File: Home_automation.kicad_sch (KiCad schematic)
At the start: 105 parts, among them Q1 BTA16-600B, Q2 BTA16-600B, Q3 BTA16-600B, Q4 BTA16-600B, Q5 BTA16-600B, Q6 BTA16-600B, SW1 SW_Push, SW2 SW_Push, U1 MOC3010M, U2 MOC3010M, U3 ESP-12E, U4 MOC3010M, U5 MOC3010M, U6 EL817, U7 MOC3010M, U8 AMS1117-3.3, U9 MOC3010M

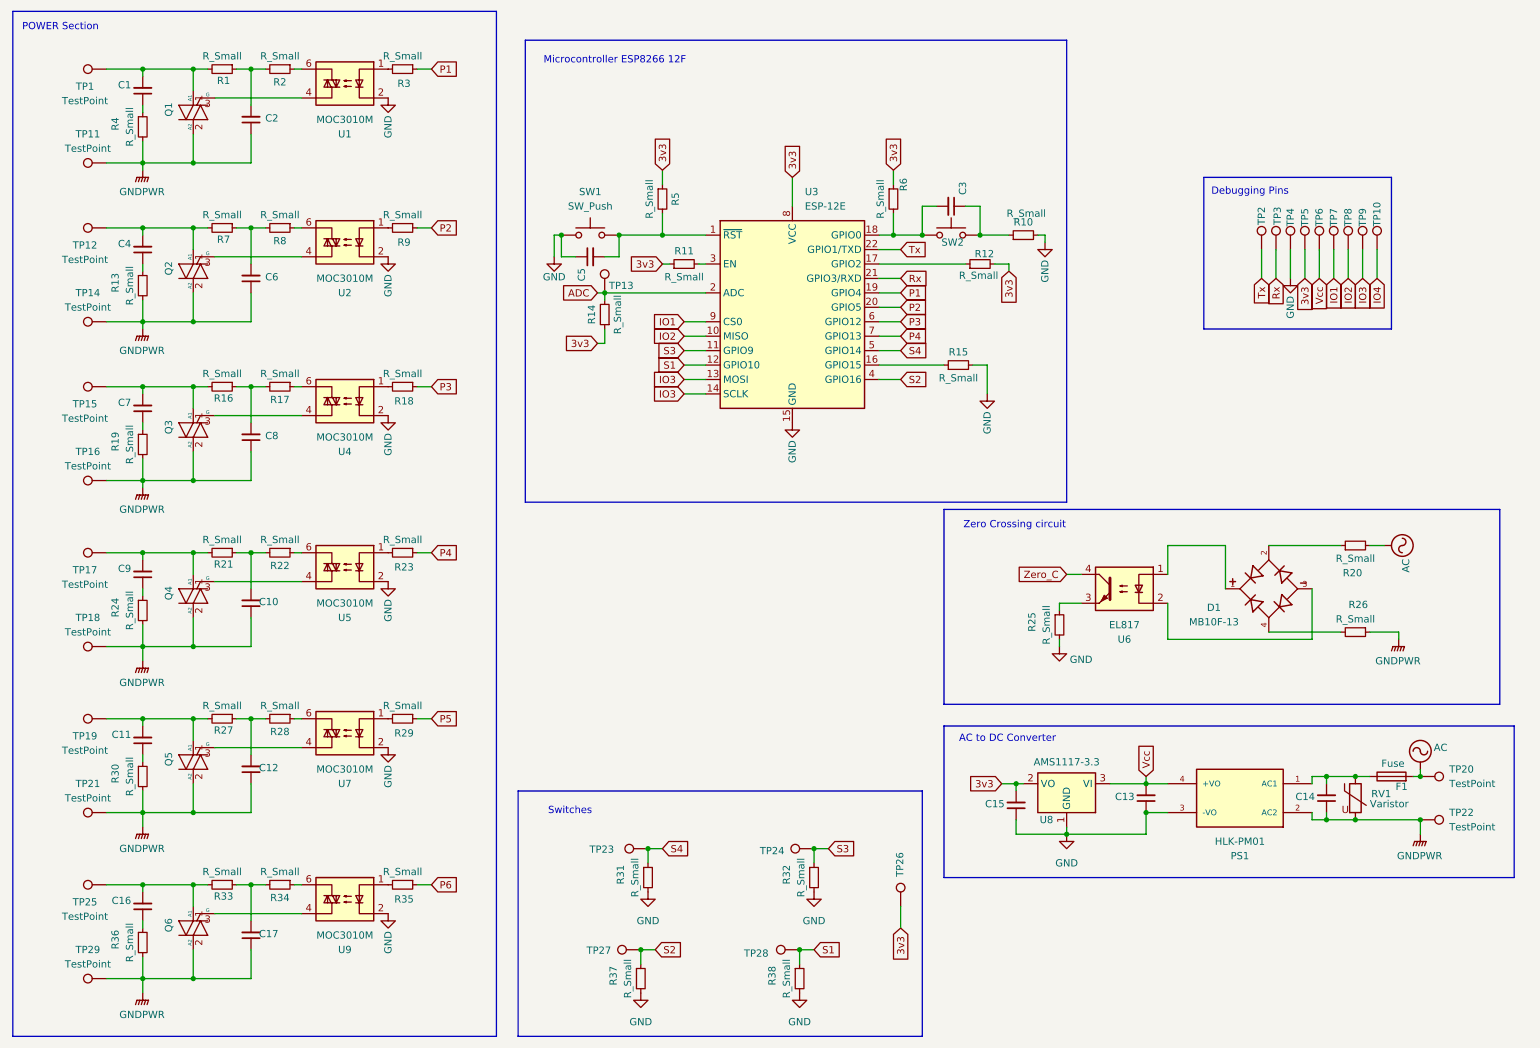
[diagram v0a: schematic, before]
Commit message: updated pcb
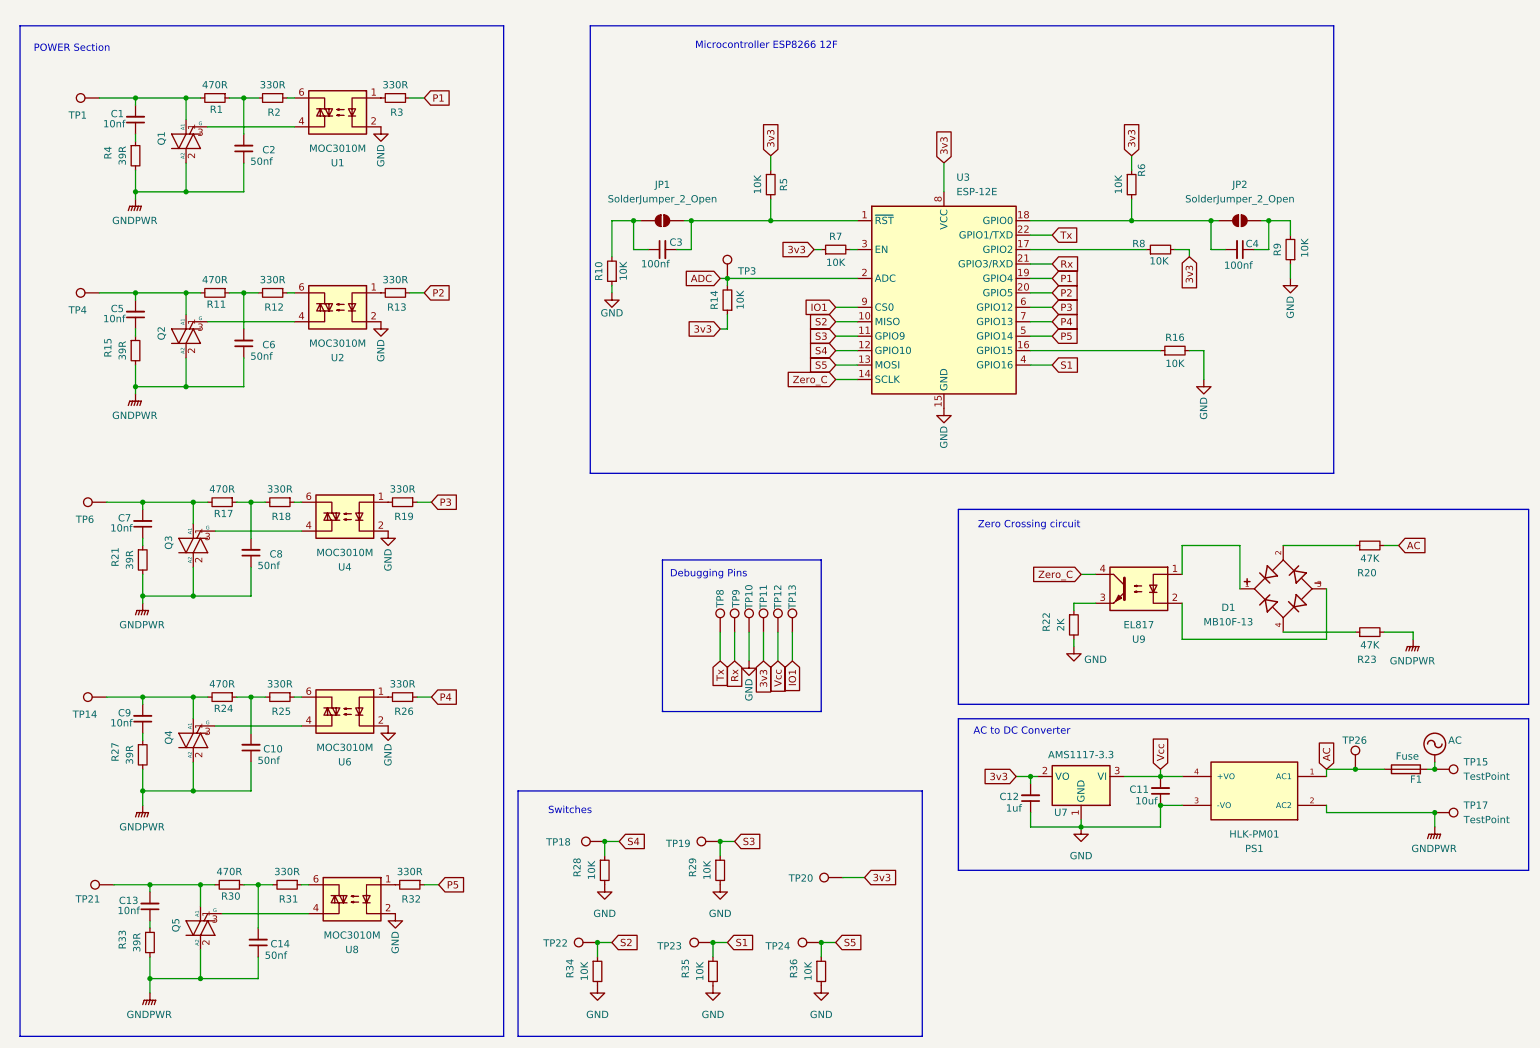
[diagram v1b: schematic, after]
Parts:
- removed C14, C16, C17, C4: C_Small, symbol Device:C_Small
- removed Q6: BTA16-600B, Package_TO_SOT_THT:TO-220-3_Vertical, symbol Triac_Thyristor:BTA16-600B
- removed R16, R22, R27, R28, R32, R37, R38, R7, R8, R9: R_Small, symbol Device:R_Small
- removed RV1: Varistor, symbol Device:Varistor
- removed SW1, SW2: SW_Push, symbol Switch:SW_Push
- removed TP10, TP11, TP14, TP16, TP18, TP21, TP25, TP29, TP8, TP9: TestPoint, symbol Connector:TestPoint
- removed U6: EL817, Package_DIP:DIP-4_W7.62mm, symbol Isolator:EL817
- removed U9: MOC3010M, symbol Relay_SolidState:MOC3010M
- added C5: 10nf, Capacitor_THT:C_Rect_L13.0mm_W3.0mm_P10.00mm_FKS3_FKP3_MKS4, symbol Device:C_Small
- added JP1, JP2: SolderJumper_2_Open, my_foot:my_foot, symbol Jumper:SolderJumper_2_Open
- added R10, R29: 10K, Resistor_SMD:R_0603_1608Metric_Pad0.98x0.95mm_HandSolder, symbol Device:R_Small
- added R11, R24: 470R, Resistor_SMD:R_0603_1608Metric_Pad0.98x0.95mm_HandSolder, symbol Device:R_Small
- added R12, R25, R31: 330R, Resistor_SMD:R_0603_1608Metric_Pad0.98x0.95mm_HandSolder, symbol Device:R_Small
- added R15: 39R, Resistor_SMD:R_0603_1608Metric_Pad0.98x0.95mm_HandSolder, symbol Device:R_Small
- added TP24, TP26: TestPoint, TestPoint:TestPoint_Loop_D3.80mm_Drill2.0mm, symbol Connector:TestPoint
- added U9: EL817, Package_DIP:DIP-4_W7.62mm, symbol Isolator:EL817
- C1, C7, C9: value C_Small -> 10nf; footprint (none) -> Capacitor_THT:C_Rect_L13.0mm_W3.0mm_P10.00mm_FKS3_FKP3_MKS4
- C10, C2, C6, C8: value C_Small -> 50nf; footprint (none) -> Capacitor_THT:C_Rect_L13.0mm_W3.0mm_P10.00mm_FKS3_FKP3_MKS4
- C11: renamed from C13; value C_Small -> 10uf; footprint (none) -> Capacitor_SMD:C_0805_2012Metric
- C12: renamed from C15; value C_Small -> 1uf; footprint (none) -> Capacitor_SMD:C_0603_1608Metric_Pad1.08x0.95mm_HandSolder
- C13: renamed from C11; value C_Small -> 10nf; footprint (none) -> Capacitor_THT:C_Rect_L13.0mm_W3.0mm_P10.00mm_FKS3_FKP3_MKS4
- C14: renamed from C12; value C_Small -> 50nf; footprint (none) -> Capacitor_THT:C_Rect_L13.0mm_W3.0mm_P10.00mm_FKS3_FKP3_MKS4
- C3: renamed from C5; value C_Small -> 100nf; footprint (none) -> Capacitor_SMD:C_0402_1005Metric_Pad0.74x0.62mm_HandSolder
- C4: renamed from C3; value C_Small -> 100nf; footprint (none) -> Capacitor_SMD:C_0402_1005Metric_Pad0.74x0.62mm_HandSolder
- F1: footprint (none) -> Fuse:Fuseholder_Cylinder-5x20mm_Schurter_0031_8201_Horizontal_Open
- R1, R17, R30: value R_Small -> 470R; footprint (none) -> Resistor_SMD:R_0603_1608Metric_Pad0.98x0.95mm_HandSolder
- R13, R18, R19, R2, R26, R3: value R_Small -> 330R; footprint (none) -> Resistor_SMD:R_0603_1608Metric_Pad0.98x0.95mm_HandSolder
- R14, R34, R35, R36, R5, R6: value R_Small -> 10K; footprint (none) -> Resistor_SMD:R_0603_1608Metric_Pad0.98x0.95mm_HandSolder
- R16: renamed from R15; value R_Small -> 10K; footprint (none) -> Resistor_SMD:R_0603_1608Metric_Pad0.98x0.95mm_HandSolder
- R20, R23: value R_Small -> 47K; footprint (none) -> Resistor_SMD:R_0603_1608Metric_Pad0.98x0.95mm_HandSolder
- R21, R33, R4: value R_Small -> 39R; footprint (none) -> Resistor_SMD:R_0603_1608Metric_Pad0.98x0.95mm_HandSolder
- R22: renamed from R25; value R_Small -> 2K; footprint (none) -> Resistor_SMD:R_0603_1608Metric_Pad0.98x0.95mm_HandSolder
- R27: renamed from R24; value R_Small -> 39R; footprint (none) -> Resistor_SMD:R_0603_1608Metric_Pad0.98x0.95mm_HandSolder
- R28: renamed from R31; value R_Small -> 10K; footprint (none) -> Resistor_SMD:R_0603_1608Metric_Pad0.98x0.95mm_HandSolder
- R32: renamed from R29; value R_Small -> 330R; footprint (none) -> Resistor_SMD:R_0603_1608Metric_Pad0.98x0.95mm_HandSolder
- R7: renamed from R11; value R_Small -> 10K; footprint (none) -> Resistor_SMD:R_0603_1608Metric_Pad0.98x0.95mm_HandSolder
- R8: renamed from R12; value R_Small -> 10K; footprint (none) -> Resistor_SMD:R_0603_1608Metric_Pad0.98x0.95mm_HandSolder
- R9: renamed from R10; value R_Small -> 10K; footprint (none) -> Resistor_SMD:R_0603_1608Metric_Pad0.98x0.95mm_HandSolder
- TP1: footprint (none) -> TestPoint:TestPoint_Loop_D3.80mm_Drill2.0mm
- TP10: renamed from TP4; footprint (none) -> TestPoint:TestPoint_Pad_1.0x1.0mm
- TP11: renamed from TP5; footprint (none) -> TestPoint:TestPoint_Pad_1.0x1.0mm
- TP12: renamed from TP6; footprint (none) -> TestPoint:TestPoint_Pad_1.0x1.0mm
- TP13: renamed from TP7; footprint (none) -> TestPoint:TestPoint_Pad_1.0x1.0mm
- TP14: renamed from TP17; footprint (none) -> TestPoint:TestPoint_Loop_D3.80mm_Drill2.0mm
- TP15: renamed from TP20; footprint (none) -> TestPoint:TestPoint_Loop_D3.80mm_Drill2.0mm
- TP17: renamed from TP22; footprint (none) -> TestPoint:TestPoint_Loop_D3.80mm_Drill2.0mm
- TP18: renamed from TP23; footprint (none) -> TestPoint:TestPoint_Loop_D3.80mm_Drill2.0mm
- TP19: renamed from TP24; footprint (none) -> TestPoint:TestPoint_Loop_D3.80mm_Drill2.0mm
- TP20: renamed from TP26; footprint (none) -> TestPoint:TestPoint_Loop_D3.80mm_Drill2.0mm
- TP21: renamed from TP19; footprint (none) -> TestPoint:TestPoint_Loop_D3.80mm_Drill2.0mm
- TP22: renamed from TP27; footprint (none) -> TestPoint:TestPoint_Loop_D3.80mm_Drill2.0mm
- TP23: renamed from TP28; footprint (none) -> TestPoint:TestPoint_Loop_D3.80mm_Drill2.0mm
- TP3: renamed from TP13; footprint (none) -> TestPoint:TestPoint_Pad_1.0x1.0mm
- TP4: renamed from TP12; footprint (none) -> TestPoint:TestPoint_Loop_D3.80mm_Drill2.0mm
- TP6: renamed from TP15; footprint (none) -> TestPoint:TestPoint_Loop_D3.80mm_Drill2.0mm
- TP8: renamed from TP2; footprint (none) -> TestPoint:TestPoint_Pad_1.0x1.0mm
- TP9: renamed from TP3; footprint (none) -> TestPoint:TestPoint_Pad_1.0x1.0mm
- U1, U2, U4: footprint (none) -> Package_DIP:DIP-6_W7.62mm
- U6: renamed from U5; footprint (none) -> Package_DIP:DIP-6_W7.62mm
- U8: renamed from U7; footprint (none) -> Package_DIP:DIP-6_W7.62mm
- renumbered U8 to U7
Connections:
- net IO2 is gone; now on net S2: U3.10 (MISO)
- net P6 is gone; now on net S1: R35.1
- net AC: now also F1.1, PS1.1 (AC1), TP26.1
- net GND: now also R34.2, R35.2, R36.2, R9.1, R10.1, R29.2; no longer C3.1, R9.2
- net GNDPWR: now also R21.2, R23.2, R33.2, R15.2; no longer R13.2, R19.2, R26.1, R30.2, R36.2
- net P2: now also R13.1
- net P3: now also R19.1; no longer R18.1
- net P4: now also R26.1; no longer R23.1
- net P5: now also U3.5 (GPIO14)
- net S1: now also U3.4 (GPIO16); no longer U3.12 (GPIO10)
- net S2: now also R34.1; no longer U3.4 (GPIO16)
- net S3: now also R29.1
- net S4: now also U3.12 (GPIO10); no longer U3.5 (GPIO14)
- net Zero_C: now also U3.14 (SCLK), U9.4
- net at R22.1: now also U9.3
- net S5: now reaches R36.1
- net S5: now also U3.13 (MOSI), TP24.1
- net at Q2.1 (A1), TP4.1: now also C5.2, R11.2
- net at C4.2, R6.2, U3.18 (GPIO0): now also JP2.1 (A)
- net at C4.1: now also R9.2, JP2.2 (B); no longer R9.1
- net at R21.1: now also C7.1; no longer C10.2
- net at C14.2: now also R30.1, R31.2
- net at C13.2, Q5.1 (A1), TP21.1: now also R30.2
- net at R17.2: now also C7.2, Q3.1 (A1), TP6.1; no longer C8.2
- net at U4.1: now also R19.2; no longer R18.2
- net at U4.6: now also R18.1; no longer R17.1
- net at C9.2, Q4.1 (A1), TP14.1: now also R24.2; no longer R21.2
- net at D1.1: now also U9.1
- net at D1.3: now also U9.2
- net at D1.4: now also R23.1; no longer R26.2
- net at C6.2: now also R11.1, R12.2
- net at C13.1: now also R33.1; no longer R30.1
- net at U6.1: now also R26.2; no longer R23.2
- net at U6.6: now also R25.1
- net at U2.6: now also R12.1
- net at C3.2, R5.2, U3.1 (~{RST}): now also JP1.2 (B)
- net at U8.6: now also R31.1
- net at U2.1: now also R13.2
- removed net IO3: U3.13 (MOSI), U3.14 (SCLK)
- new net: C10.2, R24.1, R25.2
- new net: C8.2, R17.1, R18.2
- new net: C5.1, R15.1
- new net: C3.1, JP1.1 (A), R10.2
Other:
- moved on the sheet: C11, C12, C13, C14, C3, C4, D1, F1, PS1, Q1, Q2, Q3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
